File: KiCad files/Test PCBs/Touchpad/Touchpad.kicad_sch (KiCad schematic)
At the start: 45 parts, among them J1 Conn_01x08_Male, J2 Conn_01x03_Male, U2 TTP223-BA6, U3 TTP223-BA6, U5 TTP223-BA6

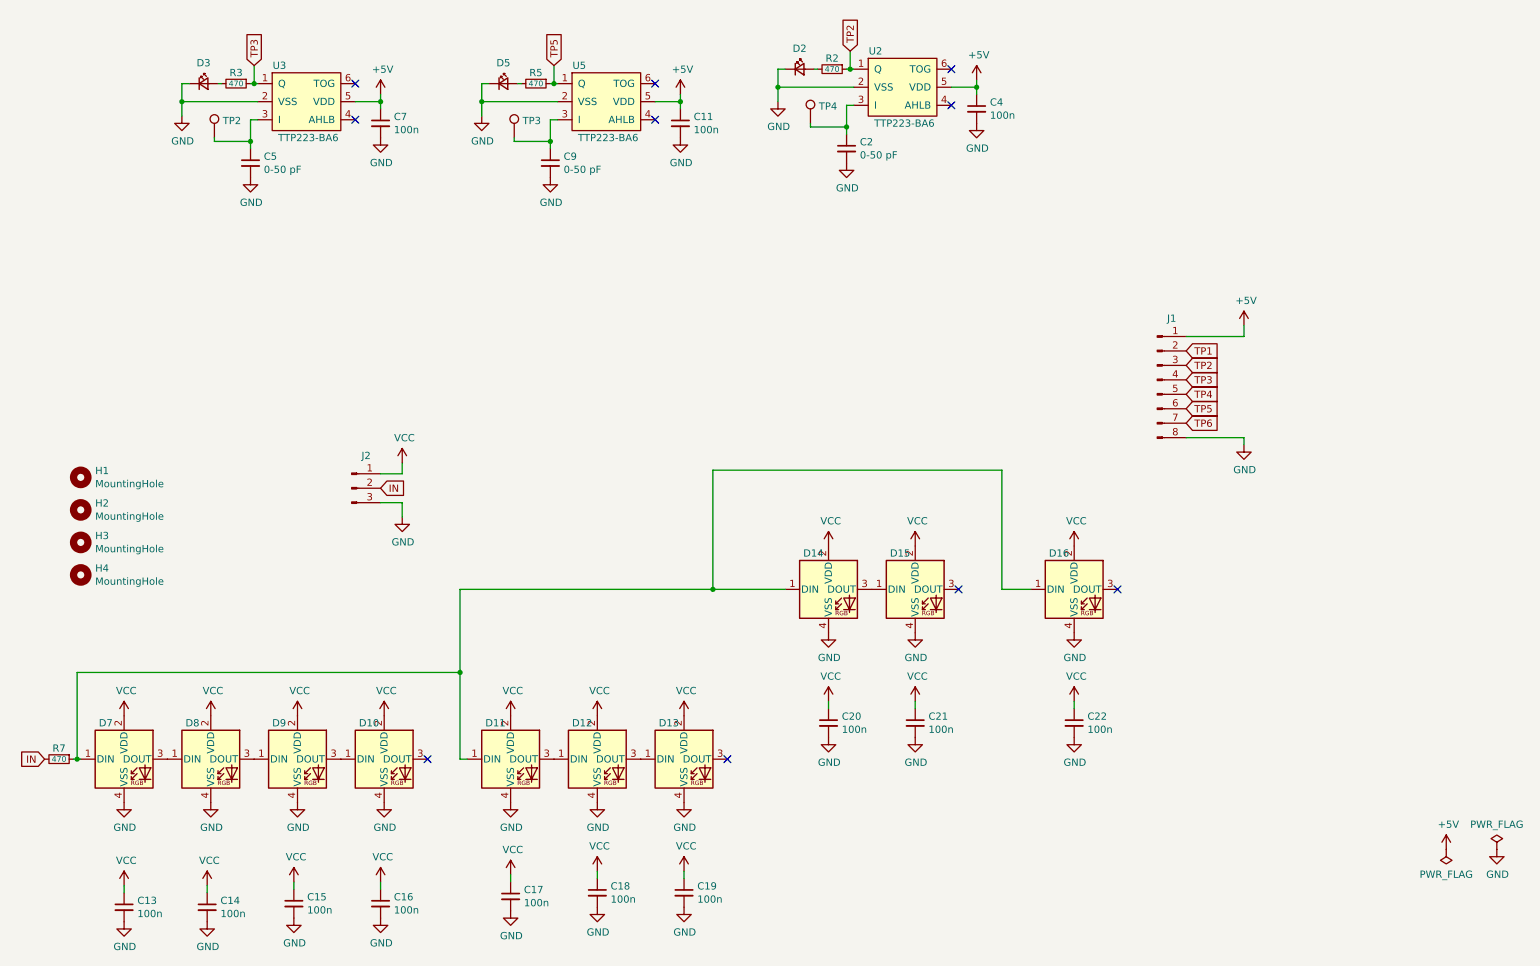
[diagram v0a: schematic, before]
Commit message: update
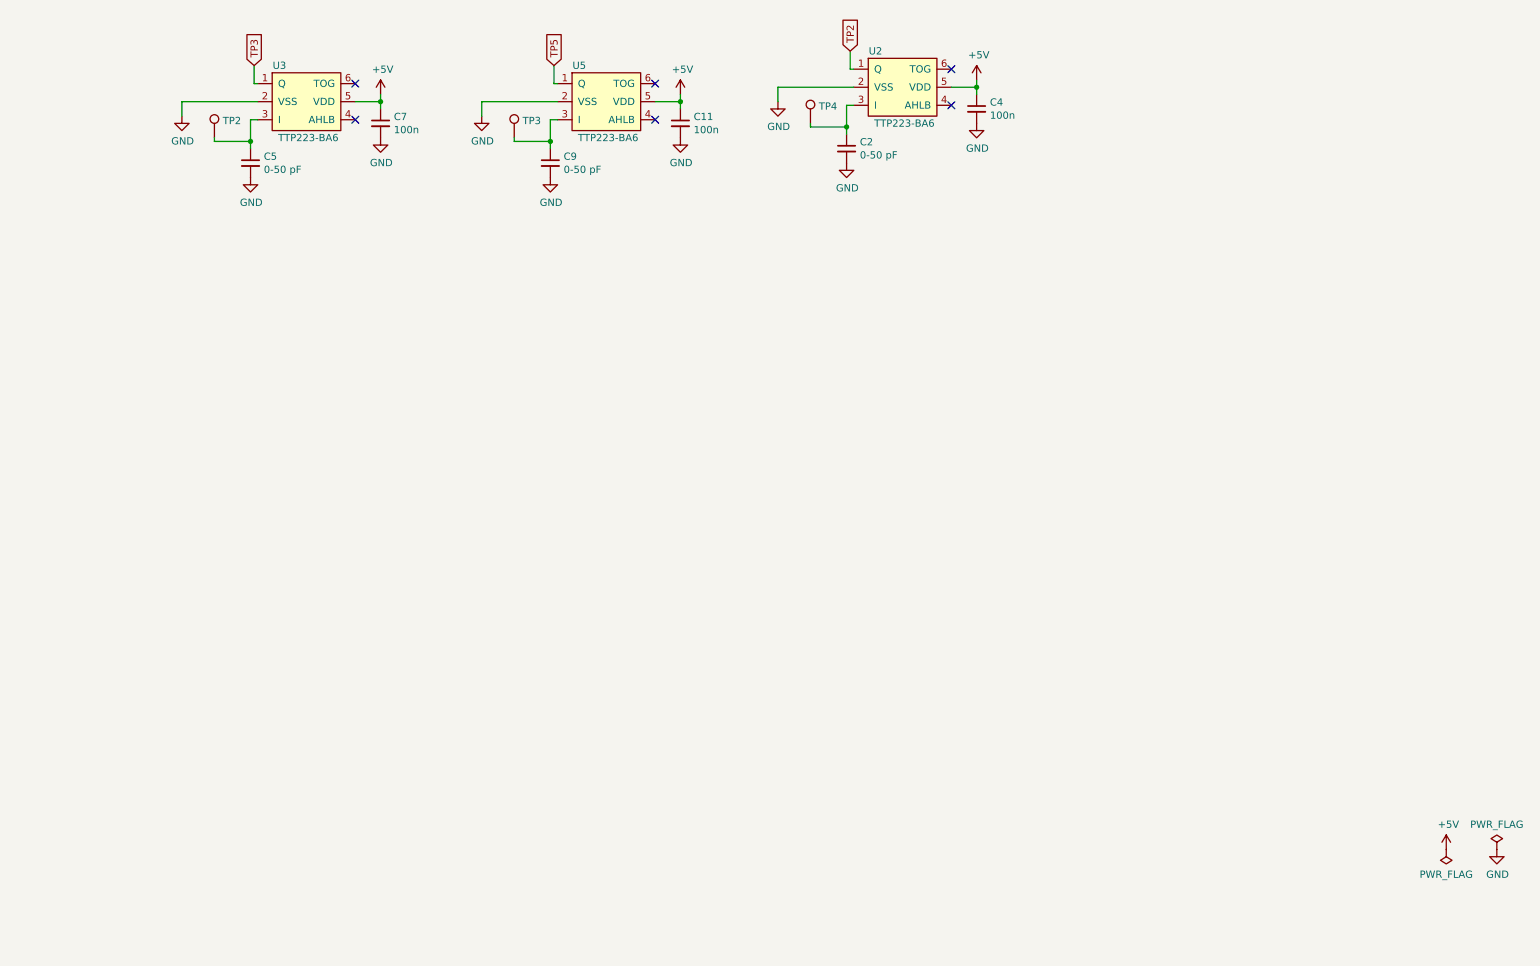
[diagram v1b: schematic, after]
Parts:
- removed C13, C14, C15, C16, C17, C18, C19, C20, C21, C22: 100n, Capacitor_SMD:C_0603_1608Metric, symbol Device:C_Small
- removed D10, D11, D12, D13, D14, D15, D16, D7, D8, D9: WS2812-4020, Touchpad:WS2812-4020, symbol ws2812-4020:WS2812-4020
- removed D2, D3, D5: LED_Small, LED_SMD:LED_0603_1608Metric, symbol Device:LED_Small
- removed H1, H2, H3, H4: MountingHole, MountingHole:MountingHole_3.2mm_M3, symbol Mechanical:MountingHole
- removed J1: Conn_01x08_Male, Connector_PinHeader_2.54mm:PinHeader_1x08_P2.54mm_Vertical, symbol Connector:Conn_01x08_Male
- removed J2: Conn_01x03_Male, Connector_PinHeader_2.54mm:PinHeader_1x03_P2.54mm_Vertical, symbol Connector:Conn_01x03_Male
- removed R2, R3, R5, R7: 470, Resistor_SMD:R_0603_1608Metric, symbol Device:R_Small
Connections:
- no-connect marks 10 -> 6
